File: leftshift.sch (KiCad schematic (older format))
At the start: 9 parts

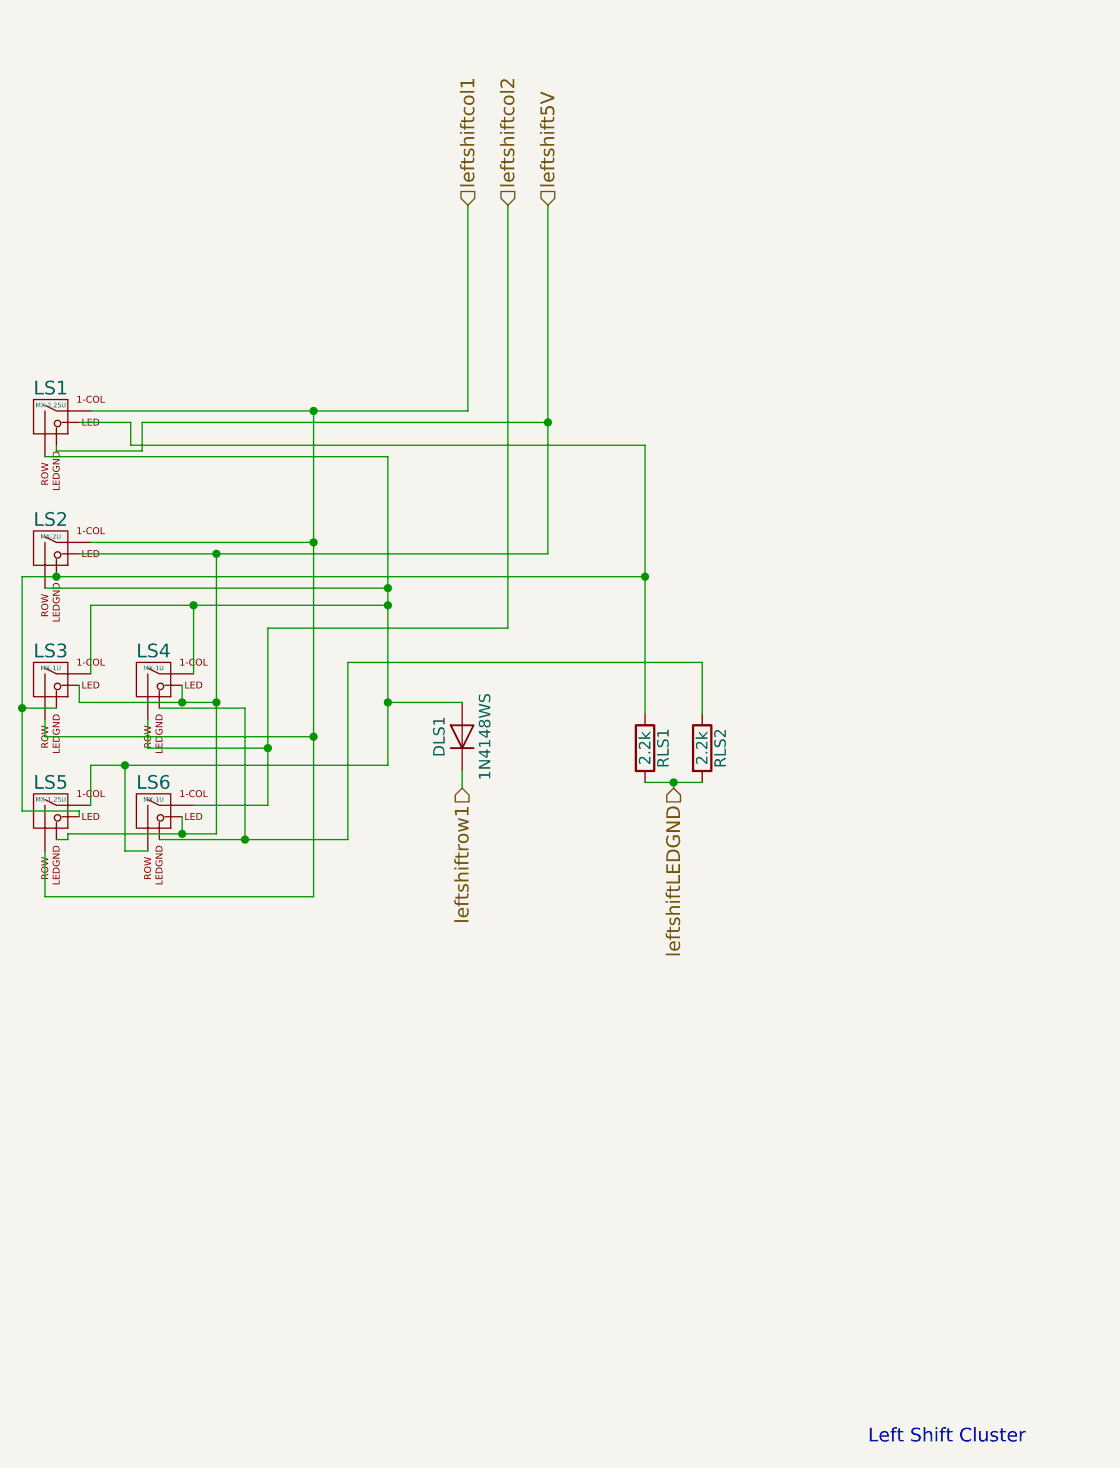
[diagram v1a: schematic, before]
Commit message: Cleaned up left shift
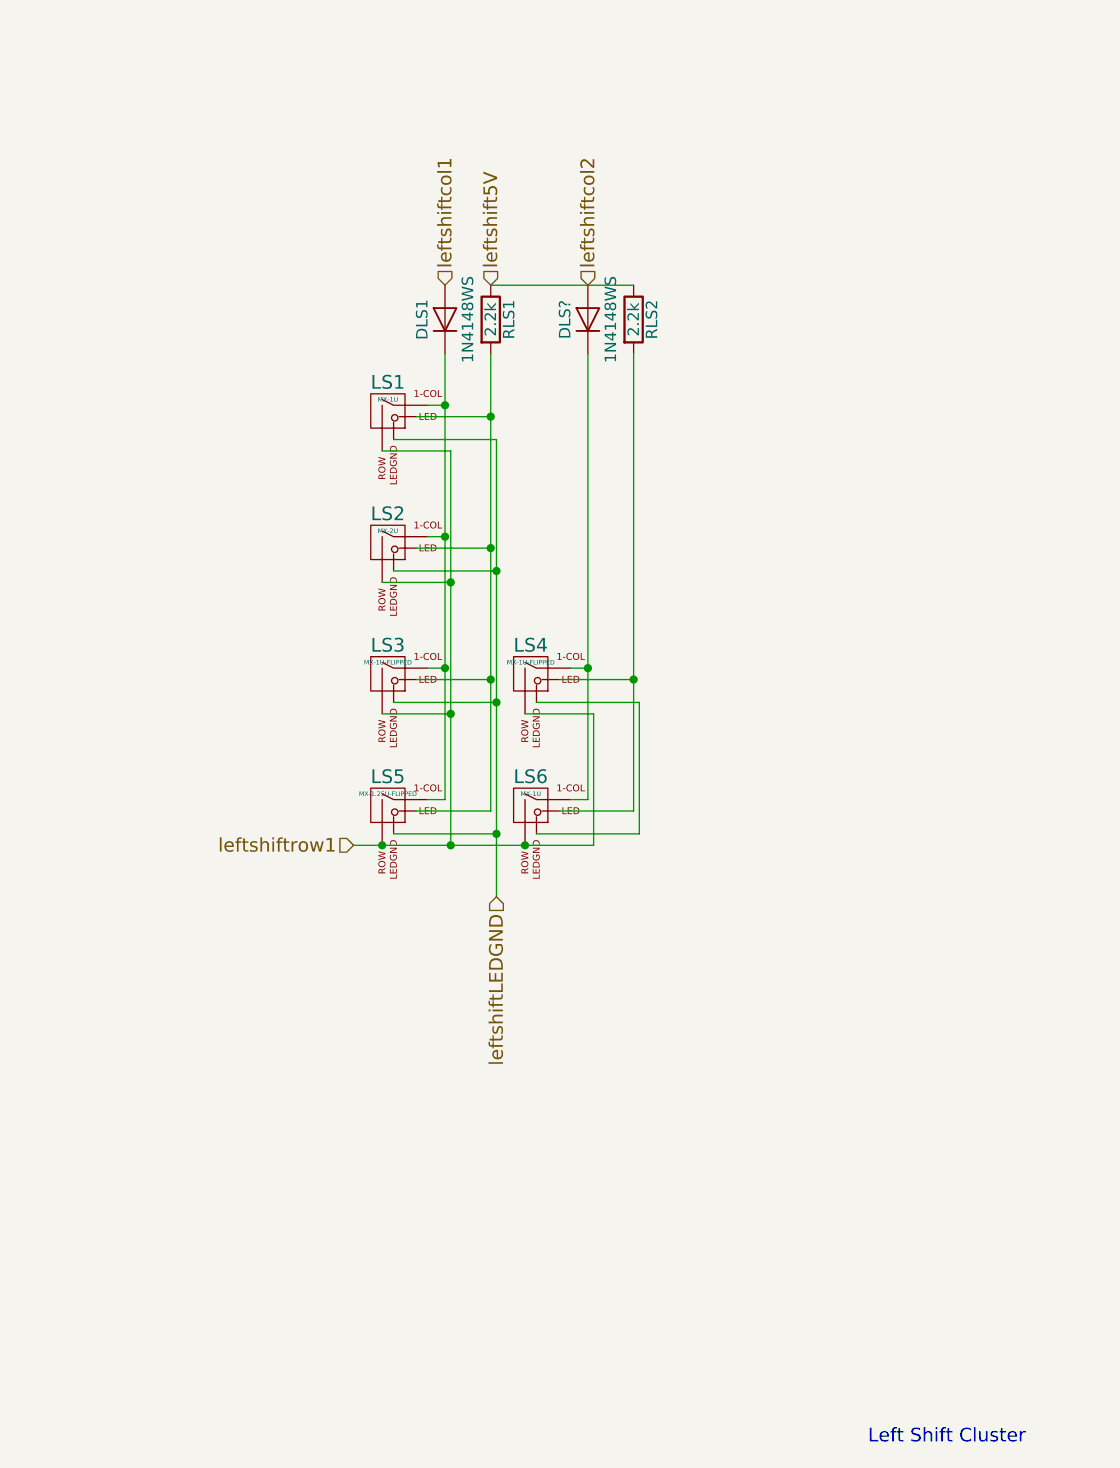
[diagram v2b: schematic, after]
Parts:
- removed LS1: MX-2.25U, symbol MX-2.25U
- removed LS3, LS4: MX-1U, symbol MX-1U
- removed LS5: MX-1.25U, symbol MX-1.25U
- added DLS?: 1N4148WS, symbol D
- added LS1: MX-1U, symbol MX-1U
- added LS3, LS4: MX-1U-FLIPPED, symbol MX-1U-FLIPPED
- added LS5: MX-1.25U-FLIPPED, symbol MX-1.25U-FLIPPED
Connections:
- net leftshift5V: now also RLS1.1, RLS2.1, DLS?.2 (A); no longer LS2.3 (LED), LS6.3 (LED)
- net leftshiftLEDGND: now also LS2.4 (LEDGND), LS1.4 (LEDGND), LS3.4 (LEDGND), LS5.4 (LEDGND); no longer RLS1.2, RLS2.2
- net leftshiftcol1: now also DLS1.2 (A); no longer LS2.1 (COL)
- net leftshiftrow1: now also LS2.2 (ROW), LS6.2 (ROW), LS1.2 (ROW), LS3.1 (ROW), LS4.1 (ROW), LS5.1 (ROW); no longer DLS1.1 (K)
- net at LS6.4 (LEDGND): now also LS4.4 (LEDGND); no longer RLS2.1
- net leftshiftcol2: no longer names the net of LS6.1 (COL)
- net leftshiftcol2: now also DLS?.1 (K), LS4.2 (COL)
- new net: DLS1.1 (K), LS1.1 (COL), LS2.1 (COL), LS3.2 (COL), LS5.2 (COL)
- new net: LS1.3 (LED), LS2.3 (LED), LS3.3 (LED), LS5.3 (LED), RLS1.2
- new net: LS4.3 (LED), LS6.3 (LED), RLS2.2
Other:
- moved on the sheet: DLS1, RLS1, RLS2
